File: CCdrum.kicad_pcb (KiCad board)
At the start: 2 copper layers, 100 x 35 mm, 31 parts, among them J1 USB_B_μ, J2 Program, J3 MIDI_out, SW1 SW_Push, SW2 SW_Push, U1 MSP430G2533, U2 AMS1117-3.3, U3 74AUP1G17

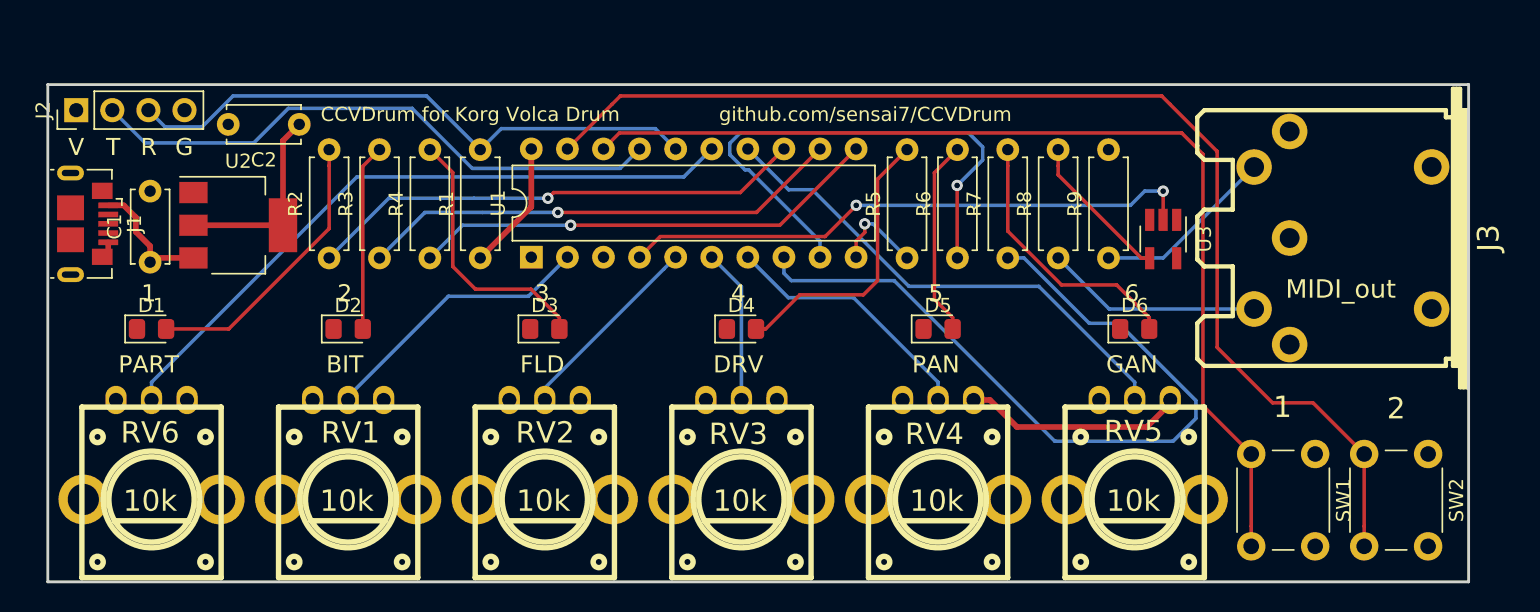
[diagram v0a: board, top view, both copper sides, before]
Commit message: New PCB design
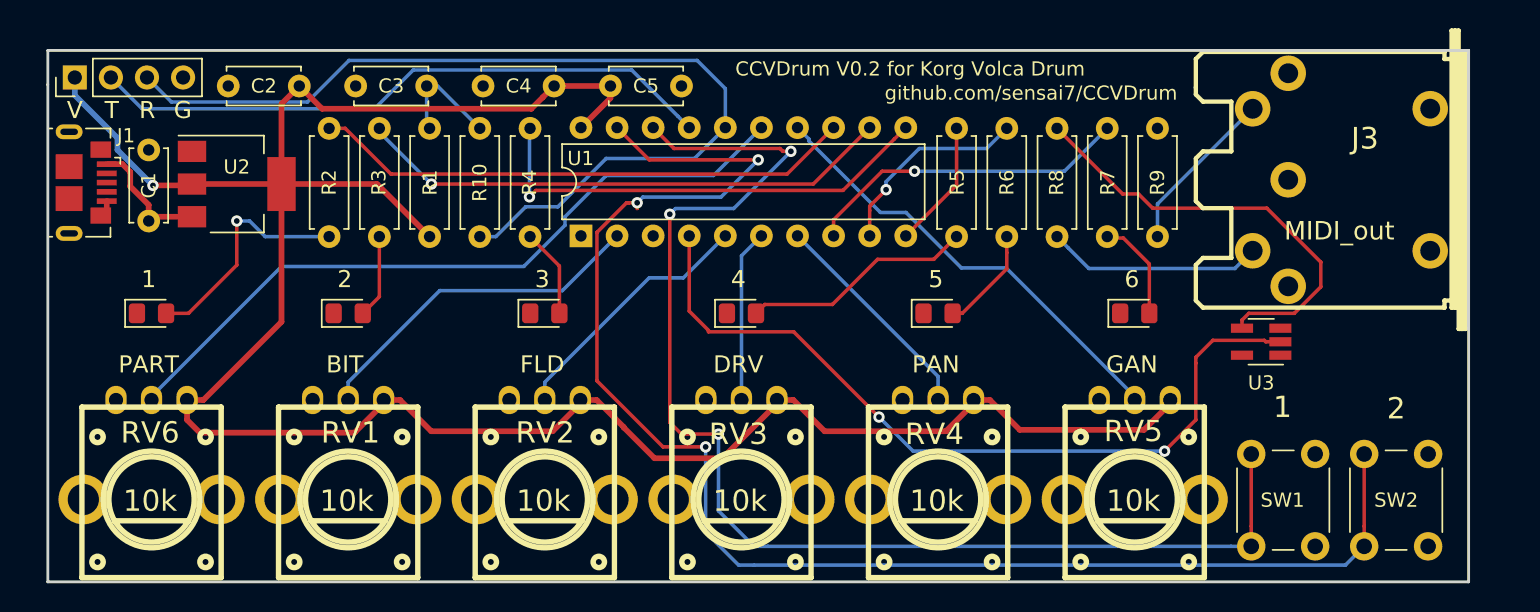
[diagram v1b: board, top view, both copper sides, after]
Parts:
- added C3: 1n, Capacitor_THT:C_Disc_D5.0mm_W2.5mm_P5.00mm, F.Cu at (56.7, 125.1)
- added C4: 10, Capacitor_THT:C_Disc_D5.0mm_W2.5mm_P5.00mm, F.Cu at (65.6, 125.1)
- added C5: 100, Capacitor_THT:C_Disc_D5.0mm_W2.5mm_P5.00mm, F.Cu at (69.6, 125.1)
- added R10: 1k, Resistor_THT:R_Axial_DIN0207_L6.3mm_D2.5mm_P7.62mm_Horizontal, F.Cu at (60.4, 135.7)
- moved R4 11.5 mm to (63.9, 128.1), turned to 270 degrees
- moved R7 11.5 mm to (104.6, 128.1), turned to 270 degrees
- moved U3 9.99 mm to (115.4, 143.1), turned to 180 degrees
- moved R5 9.76 mm to (94.0, 128.1), turned to 270 degrees
- moved R6 9.76 mm to (97.5, 128.1), turned to 270 degrees
- moved R3 9.12 mm to (53.3, 128.1), turned to 270 degrees
- moved R2 9.12 mm to (49.8, 128.1), turned to 270 degrees
- moved J3 4.10 mm to (120.3, 131.7)
- moved R1 3.87 mm to (56.9, 135.7)
- moved U1 3.80 mm to (67.5, 135.7)
- moved R9 3.76 mm to (108.1, 135.7)
- moved C1 2.90 mm to (37.1, 134.6)
- moved U2 2.90 mm to (43.3, 132.0)
- moved J1 2.90 mm to (32.7, 131.9)
- moved C2 2.70 mm to (47.7, 125.1)
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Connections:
- R1 pad 2: RST -> Net-(C3-Pad1)
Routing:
- net +3V3: track 38.6 -> 165.4 mm, vias 0 -> 1
- net LED_P6: track 54.3 -> 23.1 mm, vias 0 -> 1
- net RST: track 41.3 -> 66.7 mm
- net LED_P5: track 37.9 -> 14.2 mm
- net PUSH_L2: track 82.6 -> 105.5 mm, vias 0 -> 3
- net Net-(R8-Pad2): track 10.6 -> 31.3 mm
- net PUSH_L1: track 72.3 -> 89.6 mm, vias 0 -> 3
- net TXD: track 40.8 -> 56.9 mm
- net Net-(D3-Pad2): track 18.7 -> 6.26 mm
- net Net-(D6-Pad2): track 19.0 -> 7.23 mm
- net Net-(C3-Pad1): track 0.00 -> 8.04 mm
- net Net-(D2-Pad2): track 13.1 -> 5.88 mm
- net Net-(D5-Pad2): track 13.8 -> 7.37 mm
- net BIT: track 19.7 -> 24.4 mm
- net FLD: track 13.9 -> 18.2 mm
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- added copper zone on B.Cu, net GND
- removed copper zone on B.Cu, net +3V3
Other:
- board size 100 x 35 mm -> 100 x 37.4 mm
- board text added: "CCVDrum V0.2 for Korg Volca Drum"
- board text added: "github.com/sensai7/CCVDrum"
- board text removed: "CCVDrum for Korg Volca Drum github.com/sensai7/CCVDrum"
